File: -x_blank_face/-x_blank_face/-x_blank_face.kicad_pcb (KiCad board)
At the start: 2 copper layers, 87 x 326.5 mm, 29 parts, among them J1 Conn_01x08_Pin, J2 Conn_01x02_Pin, J3 Conn_01x02_Pin

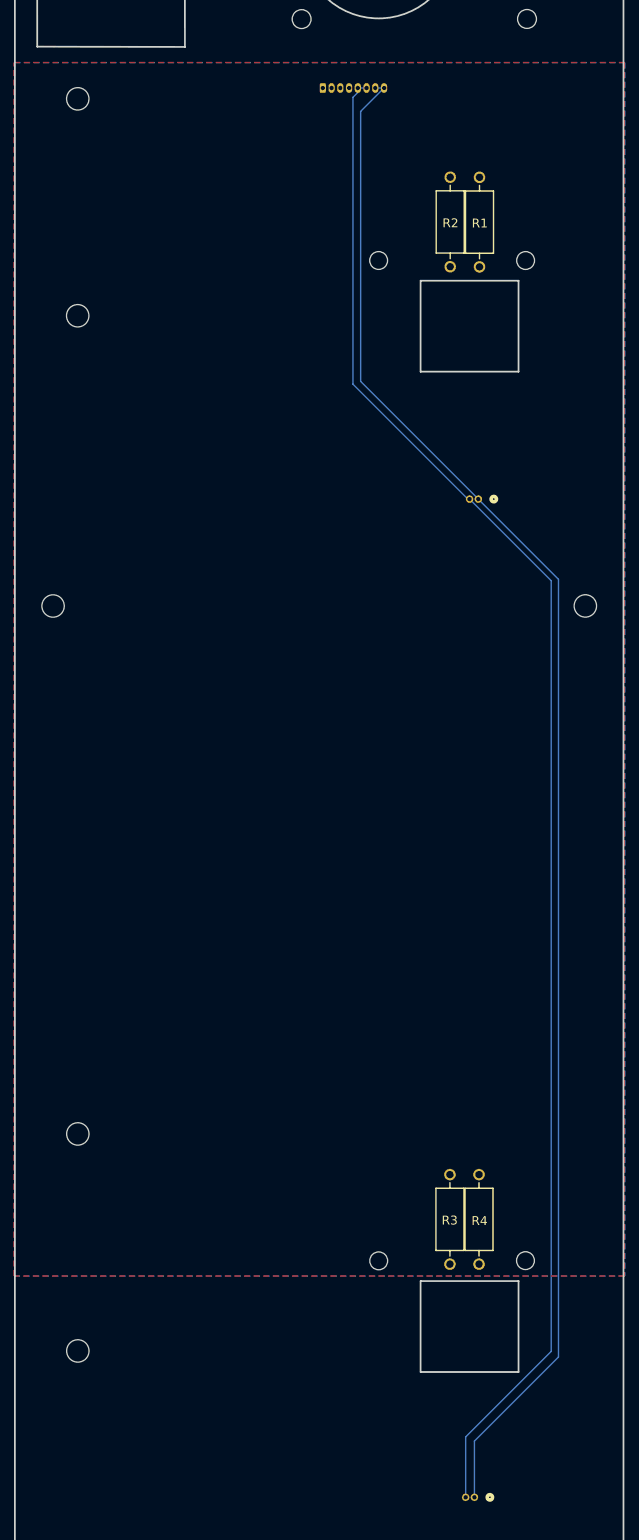
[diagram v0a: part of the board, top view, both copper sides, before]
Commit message: I forgot what I changed
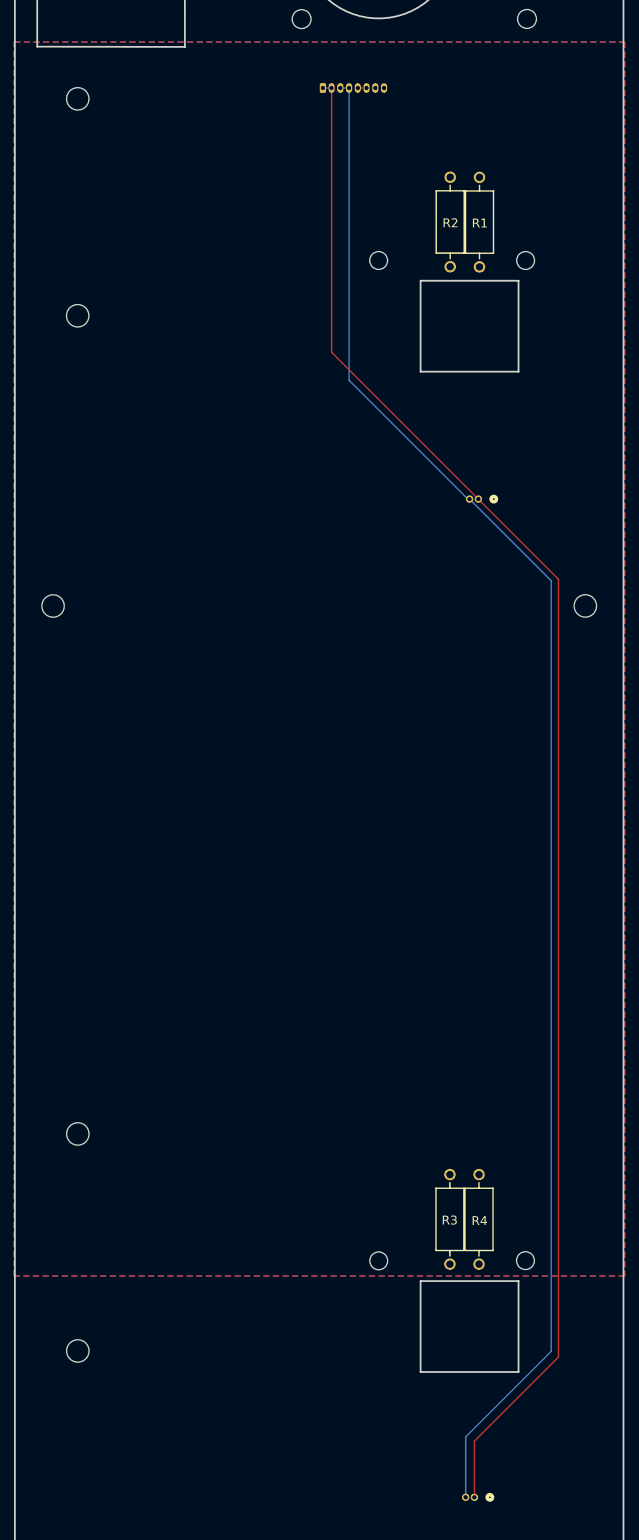
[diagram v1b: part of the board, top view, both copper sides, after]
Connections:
- J1 pad 1: /12VPDM -> GND
- J1 pad 2: /12VPDM -> GND
- J1 pad 3: /+X Drain -> /-X Serial Out
- J1 pad 4: /+X Drain -> /-X Serial Out
- J1 pad 5: /-X Serial Out -> /+X Drain
- J1 pad 6: /-X Serial Out -> /+X Drain
- J1 pad 7: GND -> /12VPDM
- J1 pad 8: GND -> /12VPDM
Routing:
- net /+X Drain: track 0.00 -> 1.89 mm
- net GND: track 220.8 -> 221.4 mm
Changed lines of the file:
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@@
 			(remove_unused_layers no)
 			(roundrect_rratio 0.25)
-			(net 4 "/12VPDM")
+			(net 1 "GND")
 			(pinfunction "Pin_1")
 			(pintype "passive")
@@
 			(layers "*.Cu" "*.Mask")
 			(remove_unused_layers no)
-			(net 4 "/12VPDM")
+			(net 1 "GND")
 			(pinfunction "Pin_2")
 			(pintype "passive")
@@
 			(layers "*.Cu" "*.Mask")
 			(remove_unused_layers no)
-			(net 2 "/+X Drain")
+			(net 3 "/-X Serial Out")
 			(pinfunction "Pin_3")
 			(pintype "passive")
@@
 			(layers "*.Cu" "*.Mask")
 			(remove_unused_layers no)
-			(net 2 "/+X Drain")
+			(net 3 "/-X Serial Out")
 			(pinfunction "Pin_4")
 			(pintype "passive")
@@
 			(layers "*.Cu" "*.Mask")
 			(remove_unused_layers no)
-			(net 3 "/-X Serial Out")
+			(net 2 "/+X Drain")
 			(pinfunction "Pin_5")
 			(pintype "passive")
@@
 			(layers "*.Cu" "*.Mask")
 			(remove_unused_layers no)
-			(net 3 "/-X Serial Out")
+			(net 2 "/+X Drain")
 			(pinfunction "Pin_6")
 			(pintype "passive")
@@
 			(layers "*.Cu" "*.Mask")
 			(remove_unused_layers no)
-			(net 1 "GND")
+			(net 4 "/12VPDM")
 			(pinfunction "Pin_7")
 			(pintype "passive")
@@
 			(layers "*.Cu" "*.Mask")
 			(remove_unused_layers no)
-			(net 1 "GND")
+			(net 4 "/12VPDM")
 			(pinfunction "Pin_8")
 			(pintype "passive")
@@
 		(end 134.7616 20.6316)
 		(width 0.2)
-		(layer "B.Cu")
-		(net 1)
-	)
-	(segment
-		(start 121.285 -38.15)
-		(end 117.936 -34.801)
-		(width 0.2)
-		(layer "B.Cu")
+		(layer "F.Cu")
 		(net 1)
 	)
@@
 		(end 134.2016 155.2784)
 		(width 0.2)
-		(layer "B.Cu")
+		(layer "F.Cu")
 		(net 1)
 	)
@@
 		(end 146.22 32.09)
 		(width 0.2)
-		(layer "B.Cu")
+		(layer "F.Cu")
 		(net 1)
 	)
@@
 		(end 146.22 143.26)
 		(width 0.2)
-		(layer "B.Cu")
+		(layer "F.Cu")
+		(net 1)
+	)
+	(segment
+		(start 113.785 -38.15)
+		(end 113.785 -0.3605)
+		(width 0.2)
+		(layer "F.Cu")
+		(net 1)
+	)
+	(segment
+		(start 113.785 -0.3605)
+		(end 134.7616 20.6161)
+		(width 0.2)
+		(layer "F.Cu")
 		(net 1)
 	)
@@
 	)
 	(segment
-		(start 117.936 3.7905)
-		(end 134.7616 20.6161)
+		(start 113.785 -38.15)
+		(end 113.785 -38.4)
 		(width 0.2)
 		(layer "B.Cu")
@@
 	)
 	(segment
-		(start 117.936 -34.801)
-		(end 117.936 3.7905)
+		(start 113.785 -38.15)
+		(end 112.535 -38.15)
 		(width 0.2)
 		(layer "B.Cu")
@@
 	)
 	(segment
-		(start 121.285 -38.15)
-		(end 120.035 -38.15)
-		(width 0.2)
-		(layer "B.Cu")
-		(net 1)
+		(start 118.785 -38.15)
+		(end 117.535 -38.15)
+		(width 0.2)
+		(layer "F.Cu")
+		(net 2)
 	)
 	(segment
 		(start 117.535 -38.15)
-		(end 118.785 -38.15)
+		(end 117.535 -37.514863)
+		(width 0.2)
+		(layer "B.Cu")
+		(net 2)
+	)
+	(segment
+		(start 116.285 3.635)
+		(end 133.2661 20.6161)
+		(width 0.2)
+		(layer "B.Cu")
+		(net 3)
+	)
+	(segment
+		(start 116.285 -38.15)
+		(end 116.285 3.635)
+		(width 0.2)
+		(layer "B.Cu")
+		(net 3)
+	)
+	(segment
+		(start 133.2661 20.6161)
+		(end 133.5116 20.6161)
+		(width 0.2)
+		(layer "B.Cu")
+		(net 3)
+	)
+	(segment
+		(start 116.285 -38.15)
+		(end 115.035 -38.15)
 		(width 0.2)
 		(layer "B.Cu")
@@
 		(start 133.5116 20.6161)
 		(end 145.18 32.2845)
-		(width 0.2)
-		(layer "B.Cu")
-		(net 3)
-	)
-	(segment
-		(start 116.840137 -36.82)
-		(end 116.840137 4.190137)
-		(width 0.2)
-		(layer "B.Cu")
-		(net 3)
-	)
-	(segment
-		(start 117.535 -37.514863)
-		(end 116.840137 -36.82)
-		(width 0.2)
-		(layer "B.Cu")
-		(net 3)
-	)
-	(segment
-		(start 117.535 -38.15)
-		(end 117.535 -37.514863)
-		(width 0.2)
-		(layer "B.Cu")
-		(net 3)
-	)
-	(segment
-		(start 116.840137 4.190137)
-		(end 133.2661 20.6161)
-		(width 0.2)
-		(layer "B.Cu")
-		(net 3)
-	)
-	(segment
-		(start 133.2661 20.6161)
-		(end 133.5116 20.6161)
 		(width 0.2)
 		(layer "B.Cu")
@@
 		(polygon
 			(pts
-				(xy 68.388089 -41.79) (xy 155.631911 -41.79) (xy 155.63722 131.68) (xy 68.38278 131.68)
+				(xy 68.388179 -44.73) (xy 155.631821 -44.73) (xy 155.63722 131.68) (xy 68.38278 131.68)
 			)
 		)
@@
 		(polygon
 			(pts
-				(xy 68.457975 -41.782627) (xy 155.701795 -41.782627) (xy 155.707104 131.687373) (xy 68.452666 131.687373)
-			)
-		)
+				(xy 68.458065 -44.722627) (xy 155.701705 -44.722627) (xy 155.707104 131.687373) (xy 68.452666 131.687373)
+			)
+		)
